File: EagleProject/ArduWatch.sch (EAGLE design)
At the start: 31 parts, among them IC1 DS1307Z, IC2 MCP73831, J1 FTS-105-01-L-D, Q1 32.768Hz, U2 ATMEGA328P-AU

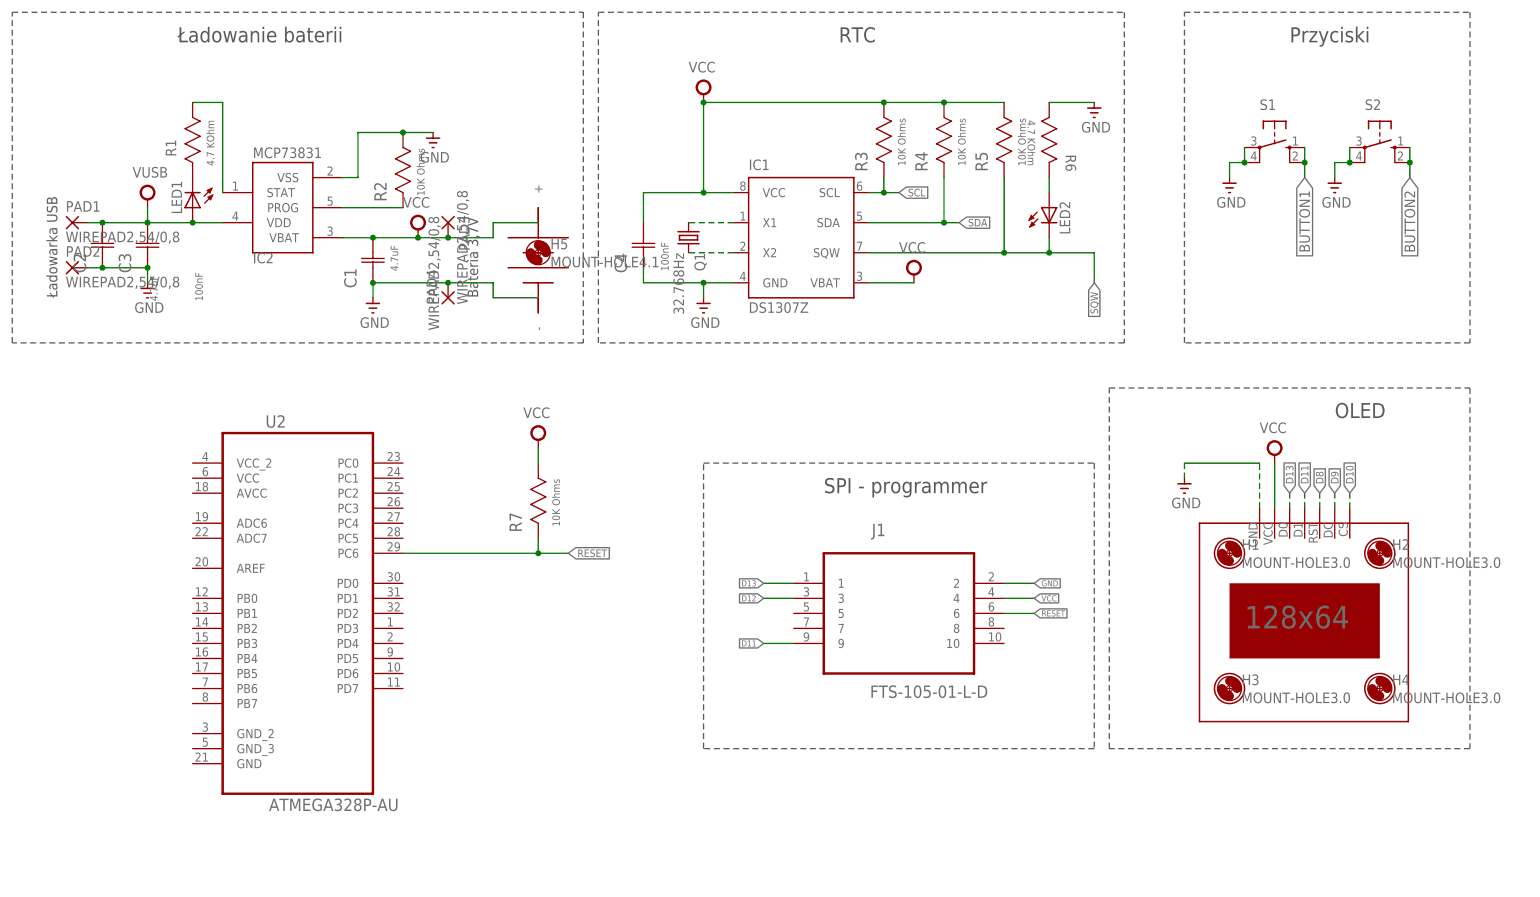
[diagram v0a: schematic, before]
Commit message: Starting Schematic
Starting Schematic in Eagle
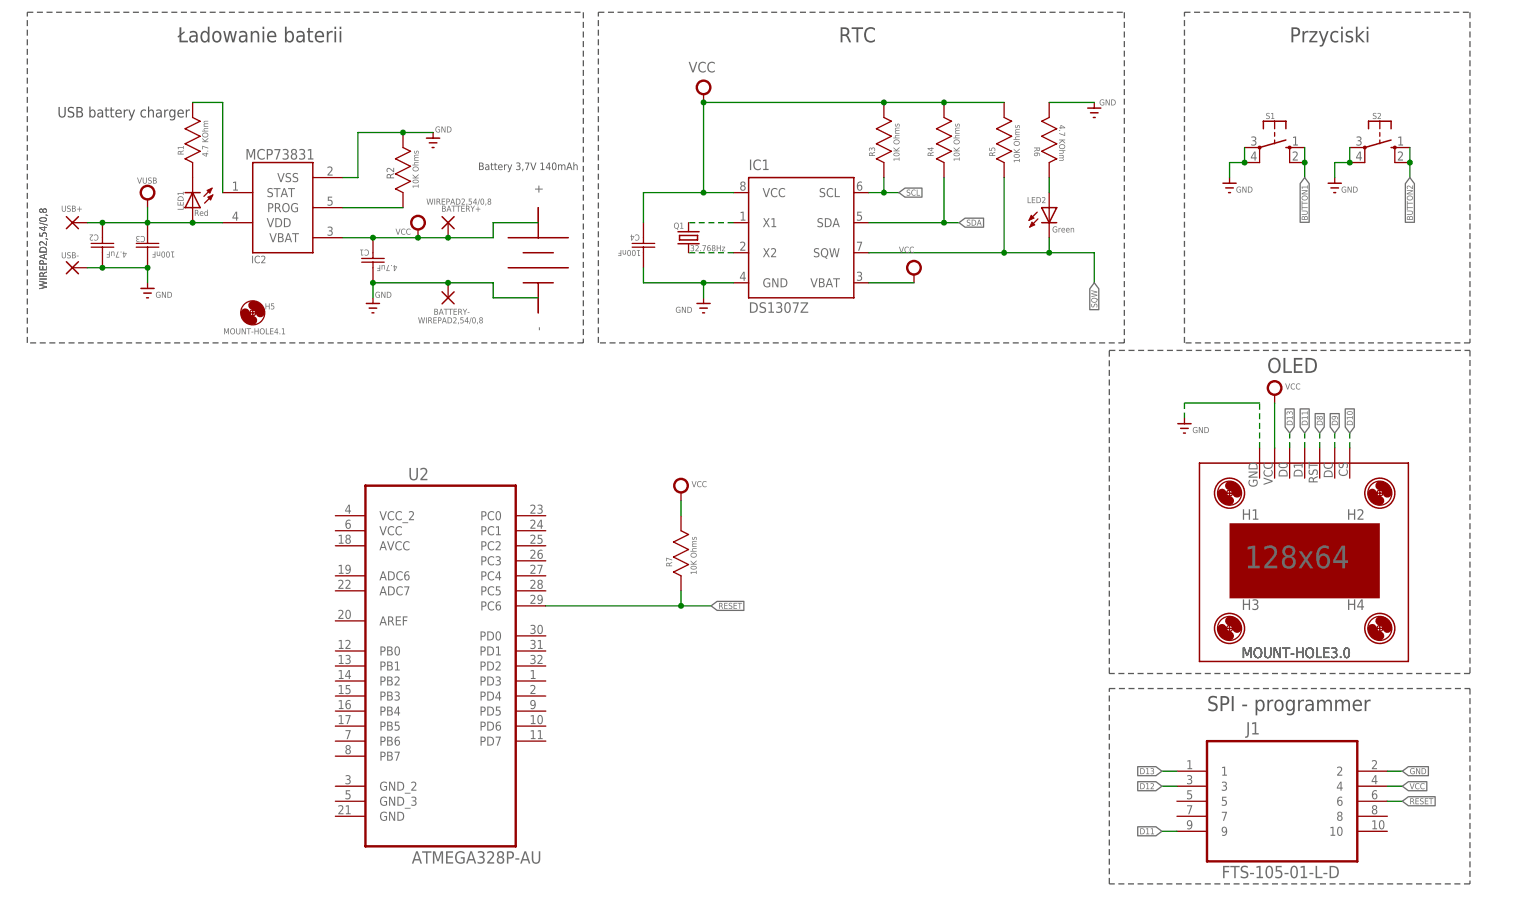
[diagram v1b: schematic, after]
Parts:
- LED1: value (none) -> Red
- LED2: value (none) -> Green
- renumbered PAD1 to USB+, PAD2 to USB-, PAD3 to BATTERY+, PAD4 to BATTERY-
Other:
- note added: "Battery 3,7V 140mAh"
- note added: "USB battery charger"
- note removed: "Bateria 3,7V"
- note removed: "Ładowarka USB"
- moved on the sheet: H1, H2, H3, H4, H5, J1, R7, U2
